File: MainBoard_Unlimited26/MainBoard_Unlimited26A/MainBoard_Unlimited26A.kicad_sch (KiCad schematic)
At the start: 38 parts, among them J1 XT, J2 Screw_Terminal_01x02, J3 BAT, J4 EN, J5 UART, J6 UART, J7 VL5, P2 SERVO, Q1 IRFZ44N, U11 ACS712xLCTR-05B, U7 ESP32-DEVKIT-V1, U8 MPU6050/BNO085 I2C, U9 AMS1117-3.3

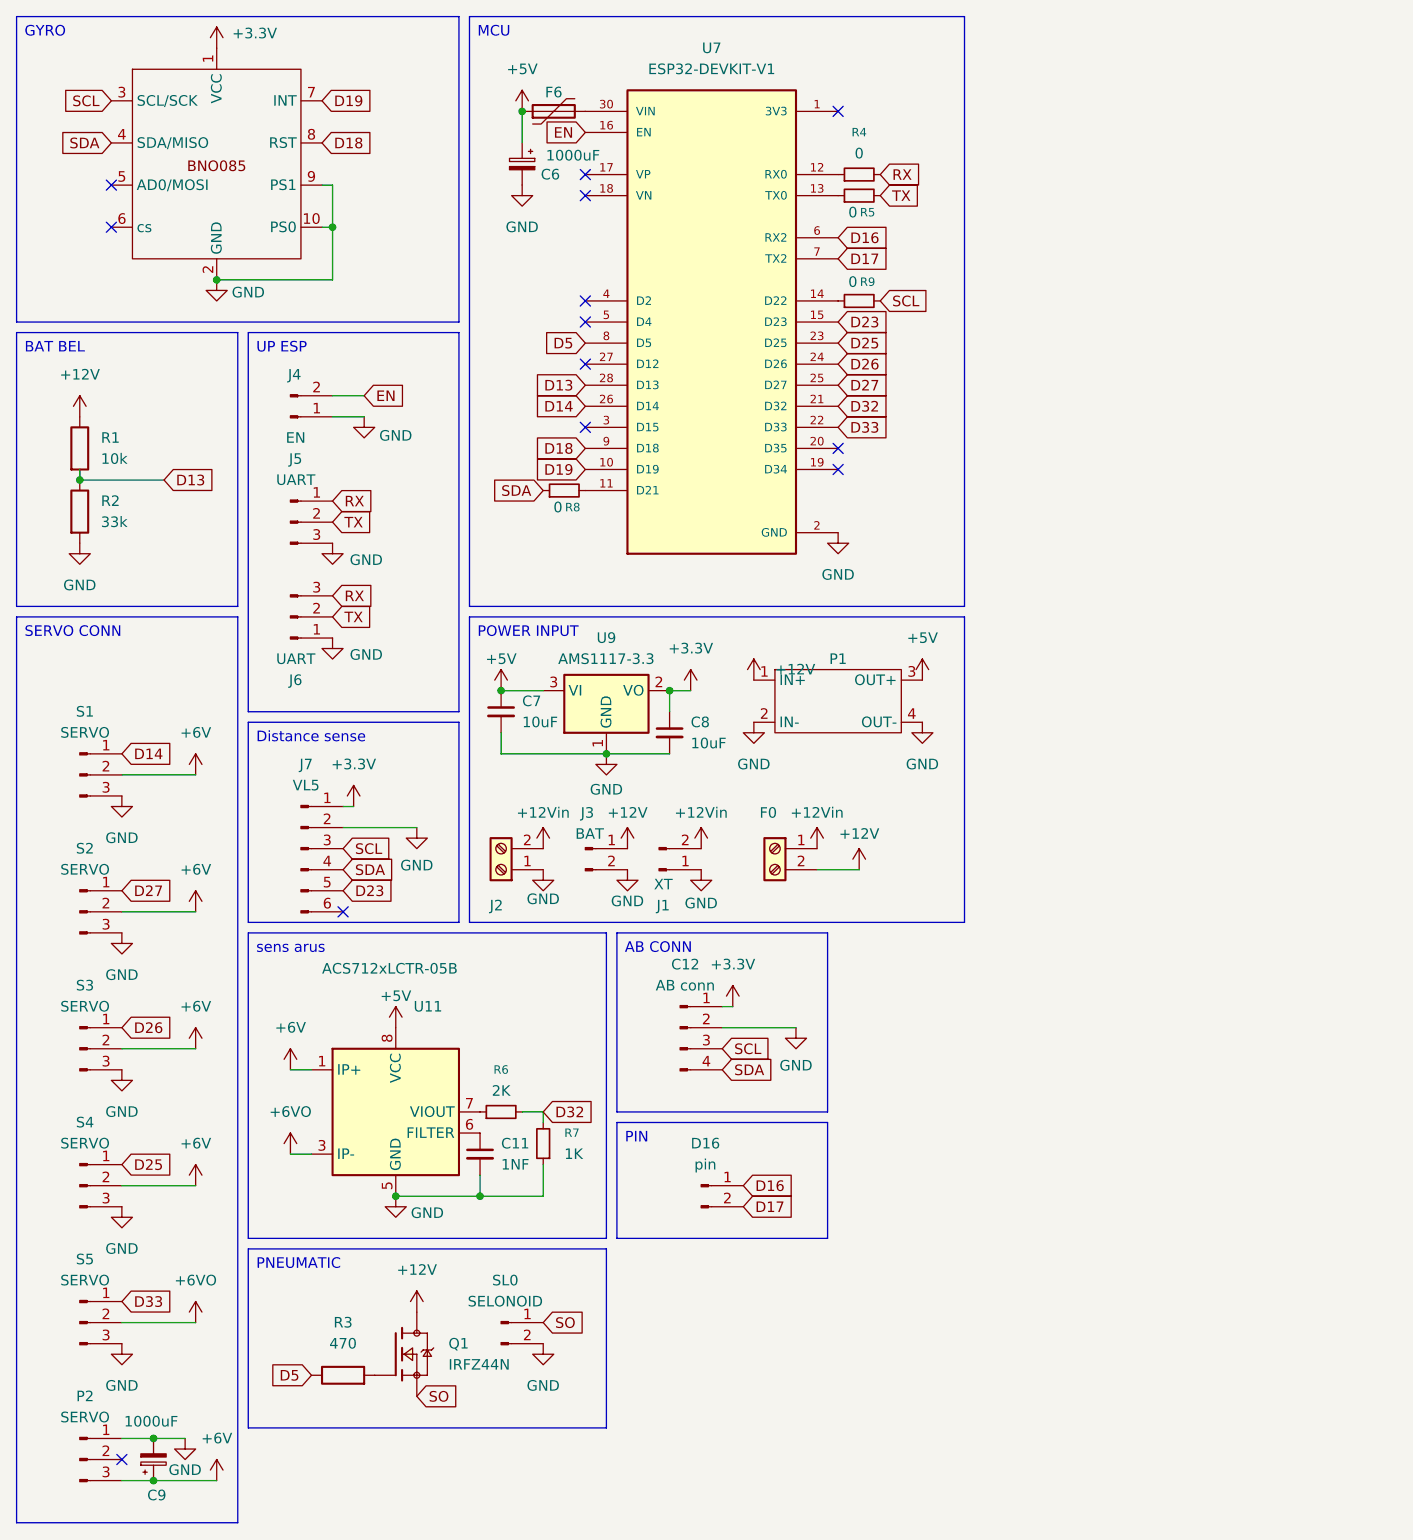
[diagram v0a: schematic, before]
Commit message: REV ALL
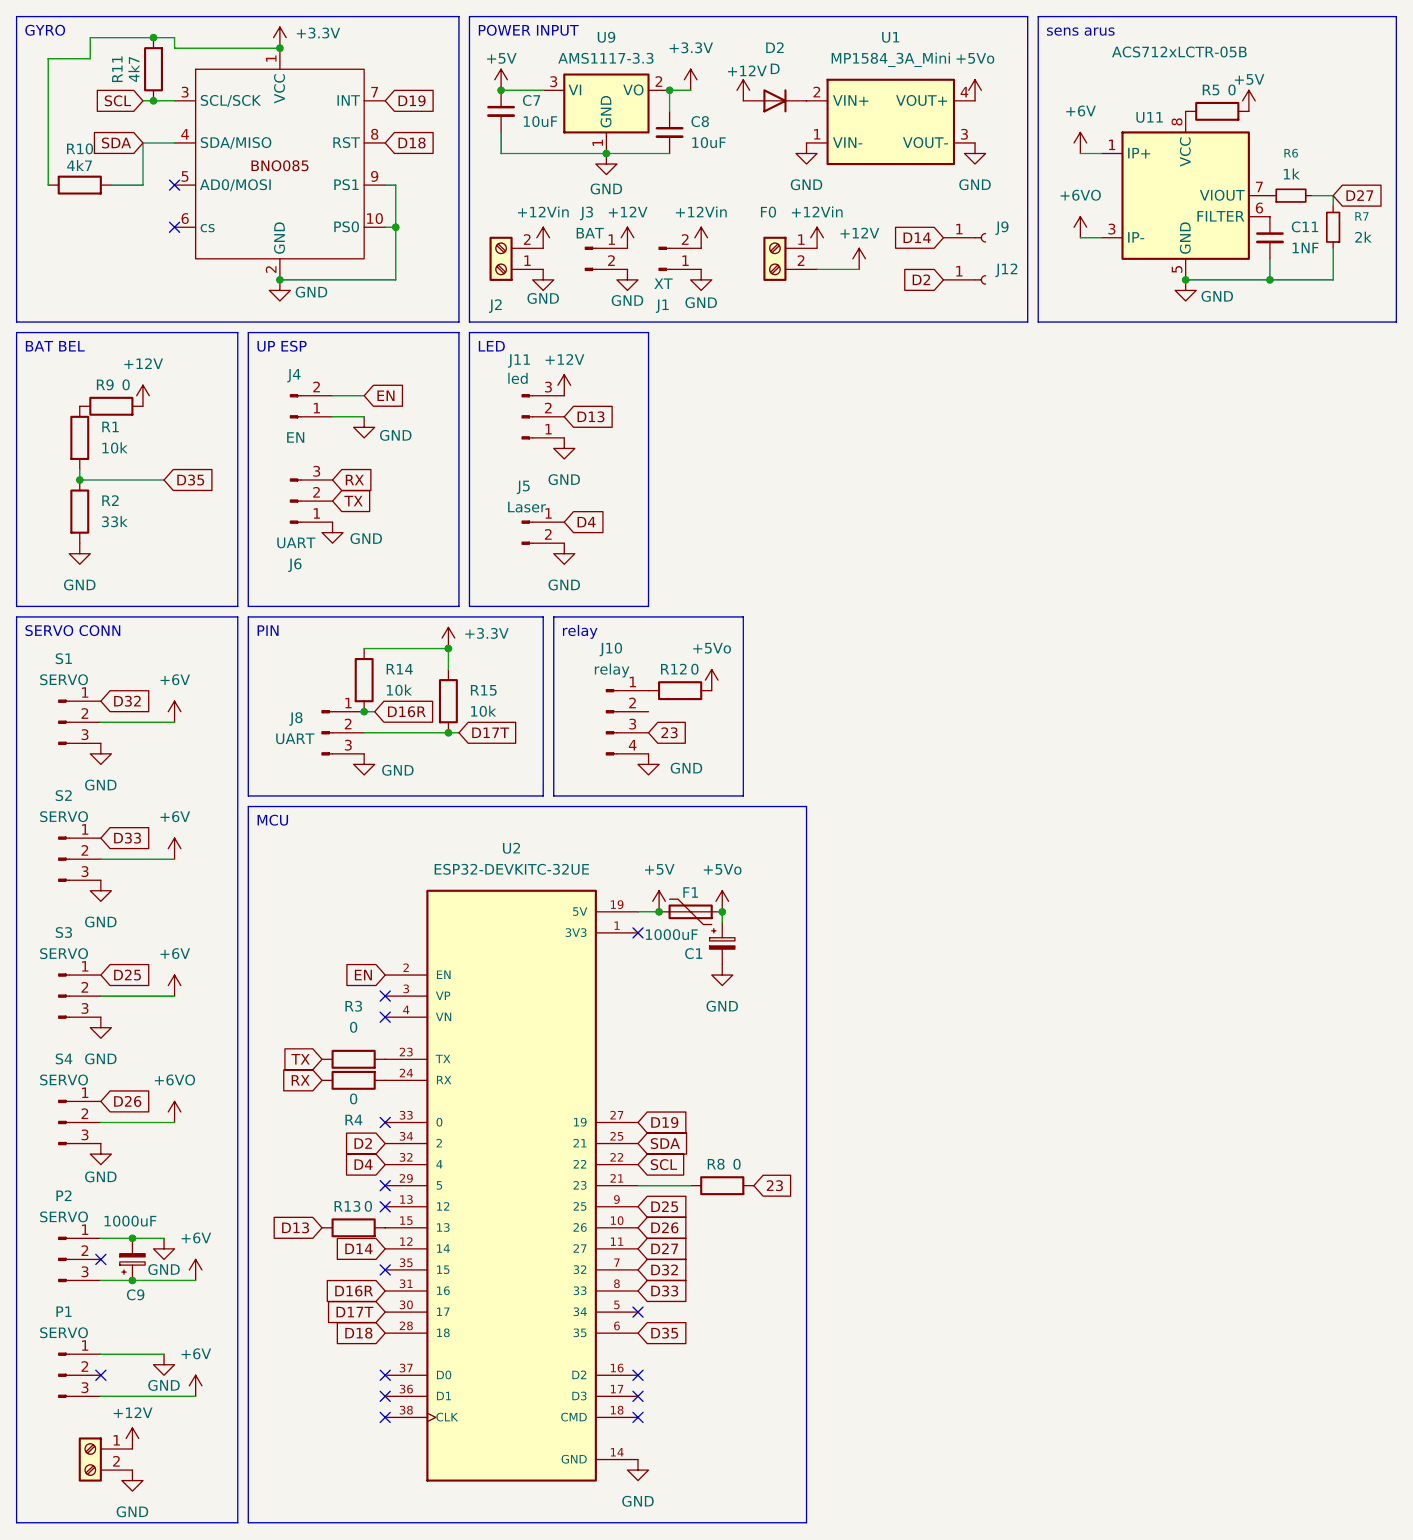
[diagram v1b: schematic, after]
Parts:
- removed C12: AB conn, Connector_JST:JST_XH_S4B-XH-A-1_1x04_P2.50mm_Horizontal, symbol Connector:Conn_01x04_Pin
- removed C6: 1000uF, Capacitor_THT:CP_Radial_D10.0mm_P5.00mm, symbol Device:C_Polarized_Small
- removed D16: pin, Connector_PinHeader_2.54mm:PinHeader_1x02_P2.54mm_Vertical, symbol Connector:Conn_01x02_Pin
- removed F6: Polyfuse, Fuse:Fuse_1812_4532Metric, symbol Device:Polyfuse
- removed J5: UART, Connector_PinHeader_2.54mm:PinHeader_1x03_P2.54mm_Horizontal, symbol Connector:Conn_01x03_Pin
- removed J7: VL5, Connector_JST:JST_XH_B6B-XH-A_1x06_P2.50mm_Vertical, symbol Connector:Conn_01x06_Pin
- removed P1: (no value), mp1548:MP1584_Module, symbol MP1584_Module:MP1584_Module_1_1
- removed Q1: IRFZ44N, IRFZ44N:TO254P1016X419X2286-3, symbol IRFZ44N:IRFZ44N
- removed R4, R5, R8, R9: 0, Resistor_SMD:R_1206_3216Metric_Pad1.30x1.75mm_HandSolder, symbol Device:R_Small
- removed S5: SERVO, Connector_JST:JST_XH_B3B-XH-A_1x03_P2.50mm_Vertical, symbol Connector:Conn_01x03_Pin
- removed SL0: SELONOID, Connector_JST:JST_XH_B2B-XH-A_1x02_P2.50mm_Vertical, symbol Connector:Conn_01x02_Pin
- removed U7: ESP32-DEVKIT-V1, ESP32-Devkit-V1:MODULE_ESP32_DEVKIT_V1, symbol ESP32:ESP32-DEVKIT-V1
- added C1: 1000uF, Capacitor_THT:CP_Radial_D10.0mm_P5.00mm, symbol Device:C_Polarized_Small
- added D2: D, Diode_SMD:D_SMA, symbol Device:D
- added F1: Polyfuse, Fuse:Fuse_1812_4532Metric, symbol Device:Polyfuse
- added J10: relay, Connector_JST:JST_XH_B4B-XH-A_1x04_P2.50mm_Vertical, symbol Connector:Conn_01x04_Pin
- added J11: led, Connector_JST:JST_XH_B3B-XH-A_1x03_P2.50mm_Vertical, symbol Connector:Conn_01x03_Pin
- added J12, J9: Conn_01x01_Socket, Connector_PinHeader_2.54mm:PinHeader_1x01_P2.54mm_Vertical, symbol Connector:Conn_01x01_Socket
- added J5: Laser, Connector_JST:JST_XH_B2B-XH-A_1x02_P2.50mm_Vertical, symbol Connector:Conn_01x02_Pin
- added J8: UART, Connector_JST:JST_XH_S3B-XH-A-1_1x03_P2.50mm_Horizontal, symbol Connector:Conn_01x03_Pin
- added P1: SERVO, Connector_JST:JST_XH_B3B-XH-A_1x03_P2.50mm_Vertical, symbol Connector:Conn_01x03_Pin
- added R10, R11: 4k7, Resistor_SMD:R_0805_2012Metric_Pad1.20x1.40mm_HandSolder, symbol Device:R
- added R12, R13, R4, R5, R8, R9: 0, Resistor_SMD:R_1206_3216Metric_Pad1.30x1.75mm_HandSolder, symbol Device:R
- added R14, R15: 10k, Resistor_SMD:R_0805_2012Metric_Pad1.20x1.40mm_HandSolder, symbol Device:R
- added S0: Screw_Terminal_01x02, TerminalBlock:TerminalBlock_MaiXu_MX126-5.0-02P_1x02_P5.00mm, symbol Connector:Screw_Terminal_01x02
- added U1: MP1584_3A_Mini, mp1548:MP1584_Module, symbol MP1584_Module:MP1584_3A_Mini
- added U2: ESP32-DEVKITC-32UE, ESP32-Devkit-V1:ESPRESSIF_ESP32-DEVKITC-32UE, symbol ESP32-DEVKITC-32UE:ESP32-DEVKITC-32UE
- J1: footprint Connector_AMASS:AMASS_XT60-M_1x02_P7.20mm_Vertical -> Connector_AMASS:AMASS_XT30U-F_1x02_P5.0mm_Vertical
- J4: footprint Connector_PinHeader_2.54mm:PinHeader_1x02_P2.54mm_Horizontal -> Connector_PinHeader_2.54mm:PinHeader_1x02_P2.54mm_Vertical
- R3: value 470 -> 0
- R6: value 2K -> 1k
- R7: value 1K -> 2k
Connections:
- net D5 is gone; now on net TX: R3.1
- net +12V: now also D2.2 (A), J11.3 (Pin_3), R9.2, S0.1 (Pin_1); no longer R1.1
- net +3.3V: now also R10.1, R11.2, R14.1, R15.1
- net +5V: now also F1.2, R5.2, U2.19 (5V); no longer U11.8 (VCC)
- net +6V: now also P1.3 (Pin_3); no longer S4.2 (Pin_2)
- net +6VO: now also S4.2 (Pin_2)
- net D13: now also J11.2 (Pin_2), R13.1; no longer R1.2, R2.1
- net D14: now also J9.1 (Pin_1), U2.12 (14); no longer S1.1 (Pin_1)
- net D18: now also U2.28 (18)
- net D19: now also U2.27 (19)
- net D25: now also S3.1 (Pin_1), U2.9 (25); no longer S4.1 (Pin_1)
- net D26: now also S4.1 (Pin_1), U2.10 (26); no longer S3.1 (Pin_1)
- net D27: now also R6.2, R7.2, U2.11 (27); no longer S2.1 (Pin_1)
- net D32: now also S1.1 (Pin_1), U2.7 (32); no longer R6.2, R7.2
- net D33: now also S2.1 (Pin_1), U2.8 (33)
- net EN: now also U2.2 (EN)
- net GND: now also C1.2, J10.4 (Pin_4), J11.1 (Pin_1), J5.2 (Pin_2), J8.3 (Pin_3), P1.1 (Pin_1), S0.2 (Pin_2), U1.1 (VIN-), U1.3 (VOUT-), U2.14 (GND), U2.20 (GND), U2.26 (GND)
- net RX: now also R4.1
- net SCL: now also R11.1, U2.22
- net SDA: now also R10.2, U2.25 (21)
- net at R3.2: now also U2.23 (TX)
- new net: J10.1 (Pin_1), R12.1
- new net: R13.2, U2.15 (13)
- new net: R8.1, U2.21 (23)
- new net: R4.2, U2.24 (RX)
- new net: R1.1, R9.1
- new net: R5.1, U11.8 (VCC)
- new net: D2.1 (K), U1.2 (VIN+)
- new net +5Vo: C1.1, F1.1, R12.2, U1.4 (VOUT+)
- new net 23: J10.3 (Pin_3), R8.2
- new net D16R: J8.1 (Pin_1), R14.2, U2.31 (16)
- new net D17T: J8.2 (Pin_2), R15.2, U2.30 (17)
- new net D2: J12.1 (Pin_1), U2.34 (2)
- new net D35: R1.2, R2.1, U2.6 (35)
- new net D4: J5.1 (Pin_1), U2.32 (4)
- no-connect marks 13 -> 18
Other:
- moved on the sheet: C11, C7, C8, C9, F0, J1, J2, J3, J6, P2, R1, R6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
